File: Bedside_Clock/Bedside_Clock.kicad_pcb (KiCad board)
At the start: 4 copper layers, 177.8 x 68.6 mm, 213 parts, among them J1 USBC_USB2.0, SW1 COLOR, SW2 MODE, SW3 BOOT, SW4 RESET, U1 ESP32-C3-MINI-1, U2 USBLC6-2SC6, U3 VCNL4040M3OE, U4 SN74LVC2T45DCTR, U5 MCP1825S

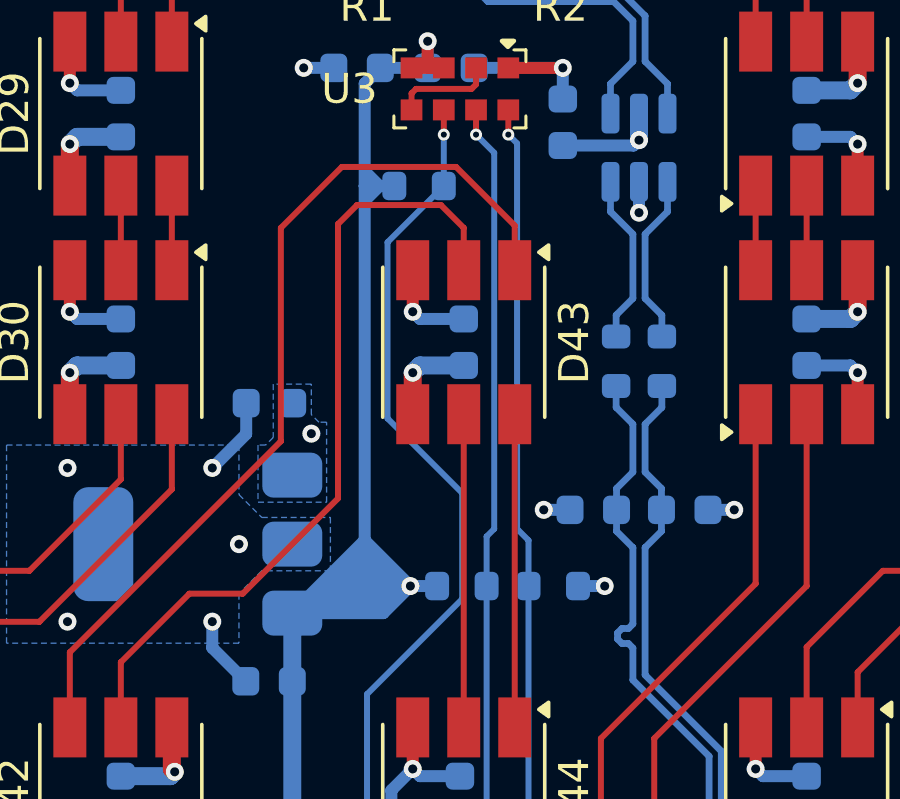
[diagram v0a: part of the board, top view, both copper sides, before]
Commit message: [Docs] Add Schematics and Renders Add Diodes, Switches, and Conns to BOM Need Resistors and Capacitors now
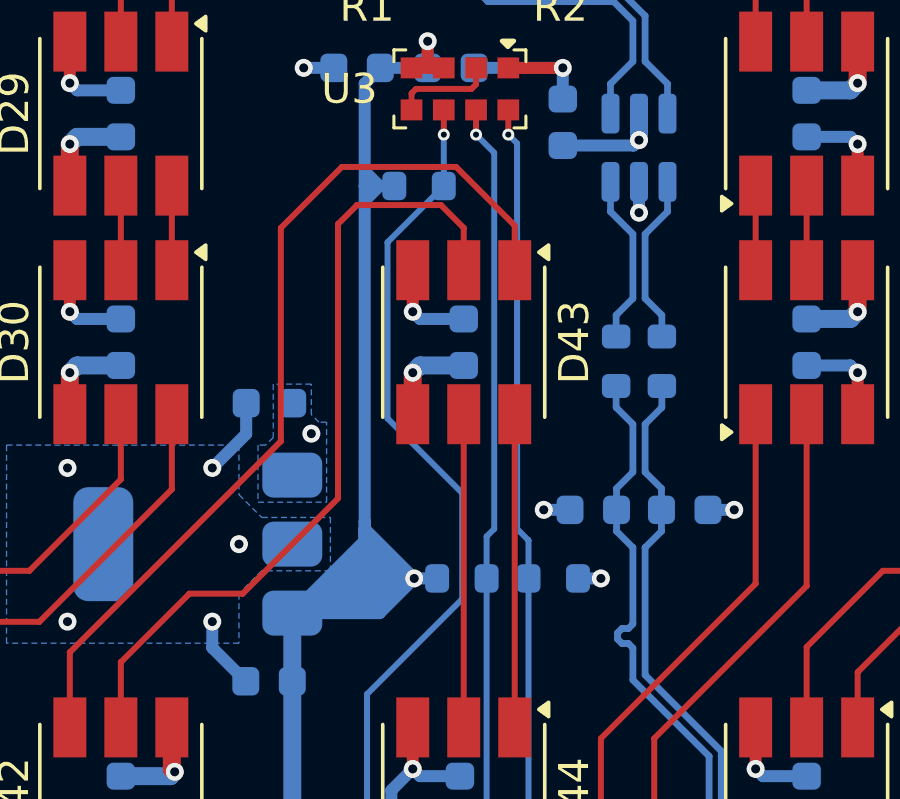
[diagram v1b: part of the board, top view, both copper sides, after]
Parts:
- R5: value 1k3 -> 1k43
- moved R10 0.25 mm to (120.6, 71.4)
- moved R11 0.25 mm to (123.6, 71.4)
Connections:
- net Net-(J1-CC2) renamed /CC2
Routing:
- net +3V3: track 83.4 -> 84.2 mm
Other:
- board text added: "3V3"
- board text added: "5V"
- board text added: "GND"
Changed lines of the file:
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@@
 	(net 186 "Net-(D87-Pad2)")
 	(net 187 "/CC1")
-	(net 188 "Net-(J1-CC2)")
+	(net 188 "/CC2")
 	(net 189 "Net-(U1-GPIO8)")
 	(net 190 "/LED_BUILTIN")
@@
 			(size 0.3 1.1)
 			(layers "F.Cu" "F.Mask" "F.Paste")
-			(net 188 "Net-(J1-CC2)")
+			(net 188 "/CC2")
 			(pinfunction "CC2")
 			(pintype "bidirectional")
@@
 			(layers "F.Cu" "F.Mask" "F.Paste")
 			(roundrect_rratio 0.25)
-			(net 188 "Net-(J1-CC2)")
+			(net 188 "/CC2")
 			(pintype "passive")
 		)
@@
 			)
 		)
-		(property "Value" "1k3"
+		(property "Value" "1k43"
 			(at 0 -1.43 90)
 			(layer "B.Fab")
@@
 	(footprint "Resistor_SMD:R_0603_1608Metric"
 		(layer "B.Cu")
-		(at 120.587 71.628 180)
+		(at 120.587 71.374 180)
 		(descr "Resistor SMD 0603 (1608 Metric), square (rectangular) end terminal, IPC-7351 nominal, (Body size source: IPC-SM-782 page 72, https://www.pcb-3d.com/wordpress/wp-content/uploads/ipc-sm-782a_amendment_1_and_2.pdf), generated with kicad-footprint-generator")
 		(tags "resistor")
@@
 	(footprint "Resistor_SMD:R_0603_1608Metric"
 		(layer "B.Cu")
-		(at 123.634 71.628)
+		(at 123.634 71.374)
 		(descr "Resistor SMD 0603 (1608 Metric), square (rectangular) end terminal, IPC-7351 nominal, (Body size source: IPC-SM-782 page 72, https://www.pcb-3d.com/wordpress/wp-content/uploads/ipc-sm-782a_amendment_1_and_2.pdf), generated with kicad-footprint-generator")
 		(tags "resistor")
@@
 		(layer "User.2")
 	)
+	(gr_text "GND"
+		(at 116.0272 70.231 0)
+		(layer "B.SilkS")
+		(effects
+			(font
+				(size 1 1)
+				(thickness 0.15)
+			)
+			(justify right mirror)
+		)
+	)
+	(gr_text "3V3"
+		(at 116.0272 72.531 0)
+		(layer "B.SilkS")
+		(effects
+			(font
+				(size 1 1)
+				(thickness 0.15)
+			)
+			(justify right mirror)
+		)
+	)
+	(gr_text "5V"
+		(at 116.0272 67.931 0)
+		(layer "B.SilkS")
+		(effects
+			(font
+				(size 1 1)
+				(thickness 0.15)
+			)
+			(justify right mirror)
+		)
+	)
 	(segment
 		(start 133.78 50.66)
@@
 	)
 	(via
-		(at 125.349 71.628)
+		(at 125.222 71.374)
 		(size 0.6)
 		(drill 0.3)
@@
 	)
 	(via
-		(at 118.872 71.628)
+		(at 118.999 71.374)
 		(size 0.6)
 		(drill 0.3)
@@
 	)
 	(segment
-		(start 118.872 71.628)
-		(end 119.762 71.628)
+		(start 117.348 69.469)
+		(end 117.348 58.293)
+		(width 0.4)
+		(layer "B.Cu")
+		(net 181)
+	)
+	(segment
+		(start 124.459 71.374)
+		(end 125.222 71.374)
+		(width 0.4)
+		(layer "B.Cu")
+		(net 181)
+	)
+	(segment
+		(start 117.348 70.118)
+		(end 117.348 69.469)
+		(width 0.4)
+		(layer "B.Cu")
+		(net 181)
+	)
+	(segment
+		(start 114.935 72.531)
+		(end 117.842 72.531)
 		(width 0.4)
 		(layer "B.Cu")
@@
 	)
 	(segment
-		(start 119.448 54.356)
-		(end 117.869 54.356)
+		(start 117.348 69.977)
+		(end 117.348 69.723)
 		(width 0.4)
 		(layer "B.Cu")
@@
 	)
 	(segment
-		(start 117.969 72.531)
-		(end 114.935 72.531)
+		(start 117.348 69.723)
+		(end 117.348 69.469)
 		(width 0.4)
 		(layer "B.Cu")
@@
 	)
 	(segment
-		(start 87.995 85.699)
-		(end 87.995 84.104)
+		(start 119.448 54.356)
+		(end 117.869 54.356)
 		(width 0.4)
 		(layer "B.Cu")
@@
 	)
 	(segment
-		(start 118.3355 58.293)
-		(end 117.348 58.293)
+		(start 114.935 72.531)
+		(end 117.348 70.118)
 		(width 0.4)
 		(layer "B.Cu")
@@
 	)
 	(segment
-		(start 118.872 71.628)
-		(end 117.969 72.531)
+		(start 119.762 71.374)
+		(end 118.999 71.374)
 		(width 0.4)
 		(layer "B.Cu")
@@
 	)
 	(segment
-		(start 114.935 79.629)
-		(end 114.935 72.531)
-		(width 0.6)
+		(start 87.995 85.699)
+		(end 87.995 84.104)
+		(width 0.4)
 		(layer "B.Cu")
 		(net 181)
 	)
 	(segment
-		(start 117.348 70.104)
-		(end 117.348 58.293)
+		(start 117.842 72.531)
+		(end 118.999 71.374)
 		(width 0.4)
 		(layer "B.Cu")
@@
 	)
 	(segment
-		(start 114.935 72.531)
-		(end 114.935 72.517)
+		(start 118.3355 58.293)
+		(end 117.348 58.293)
 		(width 0.4)
 		(layer "B.Cu")
@@
 	)
 	(segment
-		(start 126.238 81.534)
-		(end 125.475 81.534)
+		(start 117.348 70.104)
+		(end 117.348 69.723)
 		(width 0.4)
 		(layer "B.Cu")
@@
 	)
 	(segment
-		(start 119.448 53.467)
-		(end 119.448 54.356)
+		(start 114.935 79.629)
+		(end 114.935 72.531)
+		(width 0.6)
+		(layer "B.Cu")
+		(net 181)
+	)
+	(segment
+		(start 114.935 72.531)
+		(end 114.935 72.517)
 		(width 0.4)
 		(layer "B.Cu")
@@
 	)
 	(segment
-		(start 125.349 71.628)
-		(end 124.459 71.628)
+		(start 126.238 81.534)
+		(end 125.475 81.534)
 		(width 0.4)
 		(layer "B.Cu")
@@
 	)
 	(segment
-		(start 118.872 71.628)
-		(end 117.348 70.104)
+		(start 119.448 53.467)
+		(end 119.448 54.356)
 		(width 0.4)
 		(layer "B.Cu")
@@
 	)
 	(segment
-		(start 114.935 72.517)
-		(end 117.348 70.104)
+		(start 117.348 54.877)
+		(end 117.869 54.356)
 		(width 0.4)
 		(layer "B.Cu")
@@
 	)
 	(segment
-		(start 117.348 54.877)
-		(end 117.869 54.356)
+		(start 118.999 71.374)
+		(end 117.348 69.723)
 		(width 0.4)
 		(layer "B.Cu")
@@
 	)
 	(segment
-		(start 125.349 71.628)
-		(end 118.872 71.628)
+		(start 125.222 71.374)
+		(end 118.999 71.374)
 		(width 0.4)
-		(layer "In2.Cu")
+		(layer "In1.Cu")
 		(net 181)
 	)
